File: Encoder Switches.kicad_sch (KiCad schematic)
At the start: 63 parts

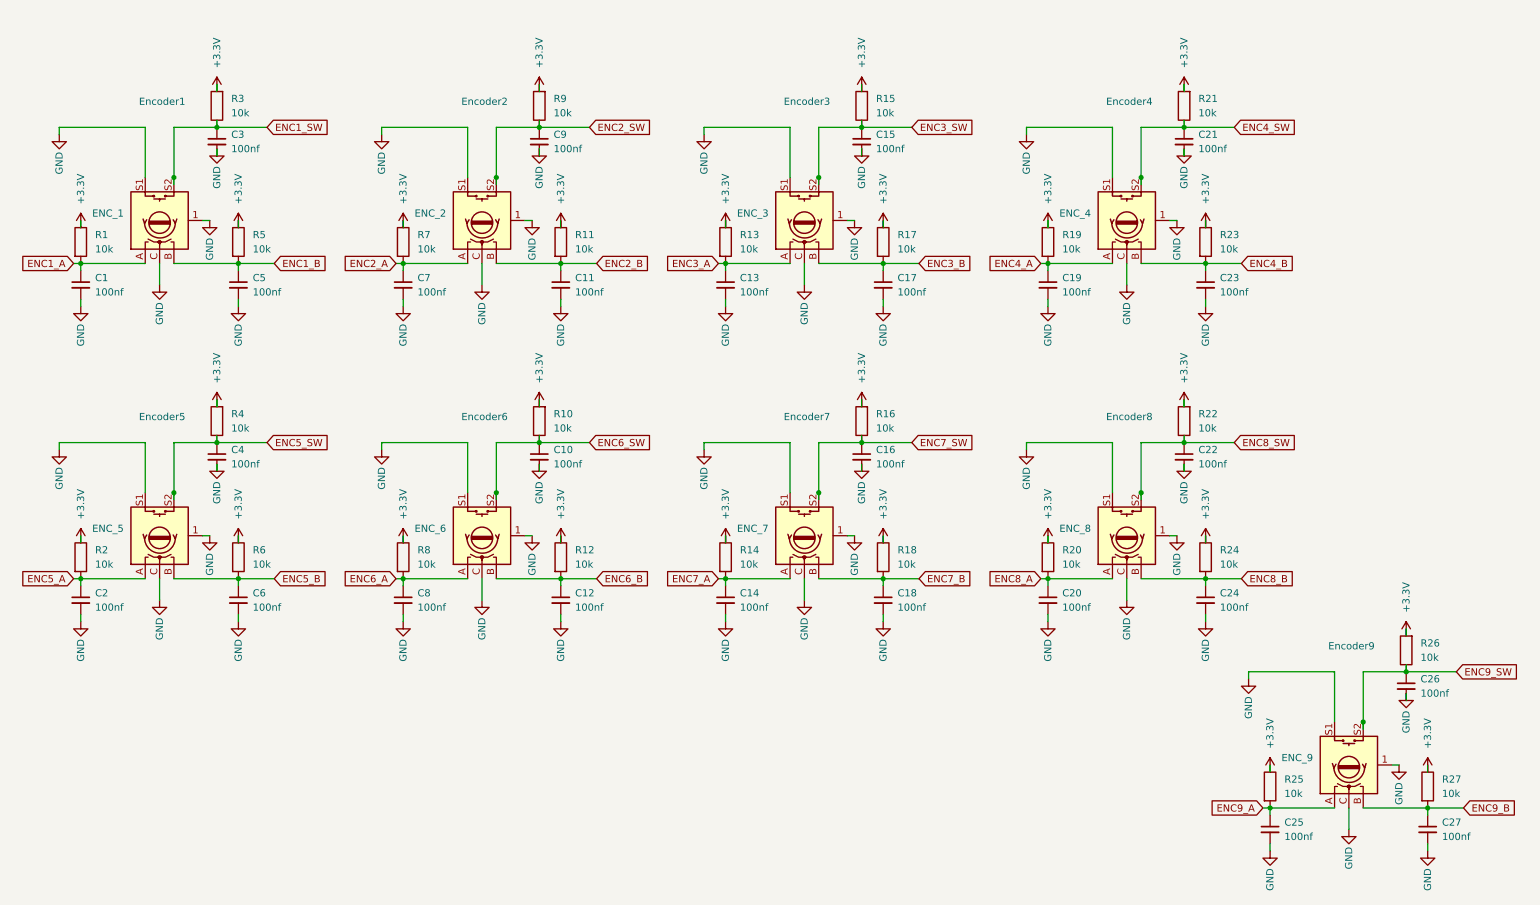
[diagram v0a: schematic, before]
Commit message: Solve all warnings
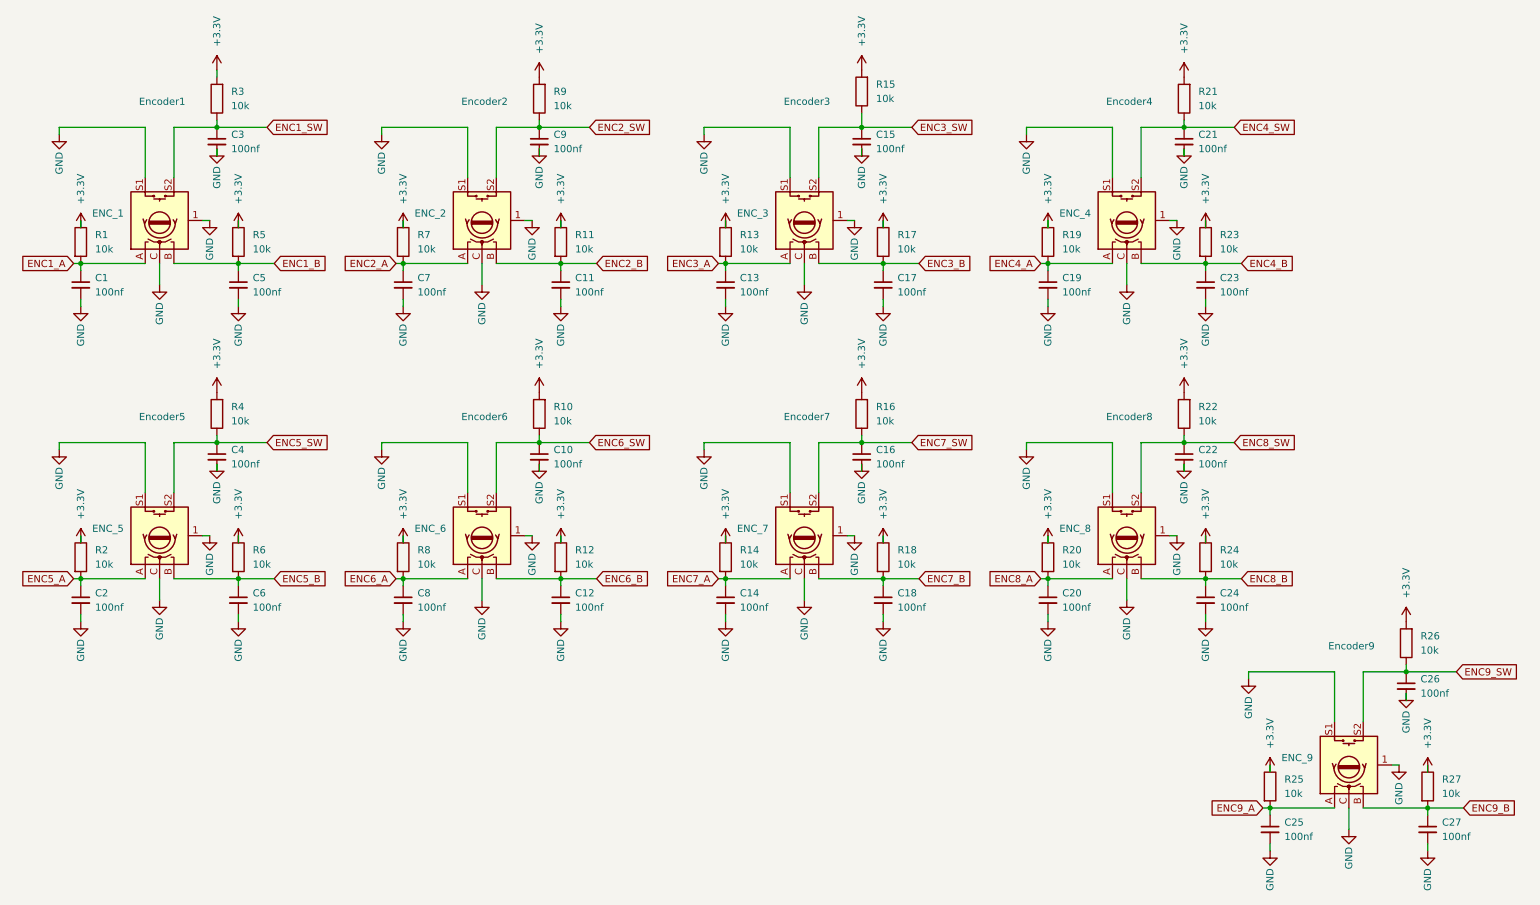
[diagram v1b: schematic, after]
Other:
- moved on the sheet: R10, R15, R16, R21, R22, R26, R3, R4, R9
